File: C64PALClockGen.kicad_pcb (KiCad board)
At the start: 2 copper layers, 21.7 x 32.7 mm, 20 parts, among them J1 Conn_01x08_Pin, J2 Conn_01x08_Pin, U1 74AHCT1G125, U2 LDL1117S33, U3 74AHCT1G125, Y1 5V49EE902

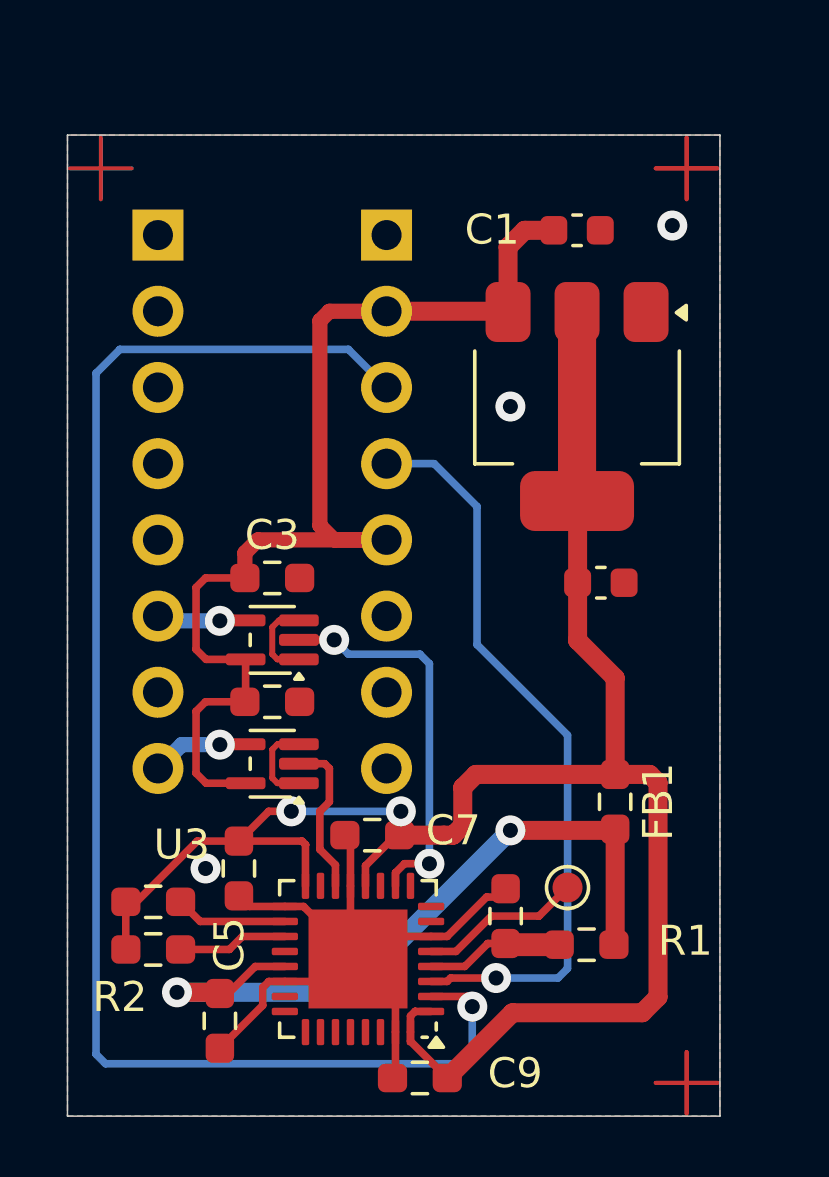
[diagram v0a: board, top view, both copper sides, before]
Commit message: C64 Clock Generator Rev.B
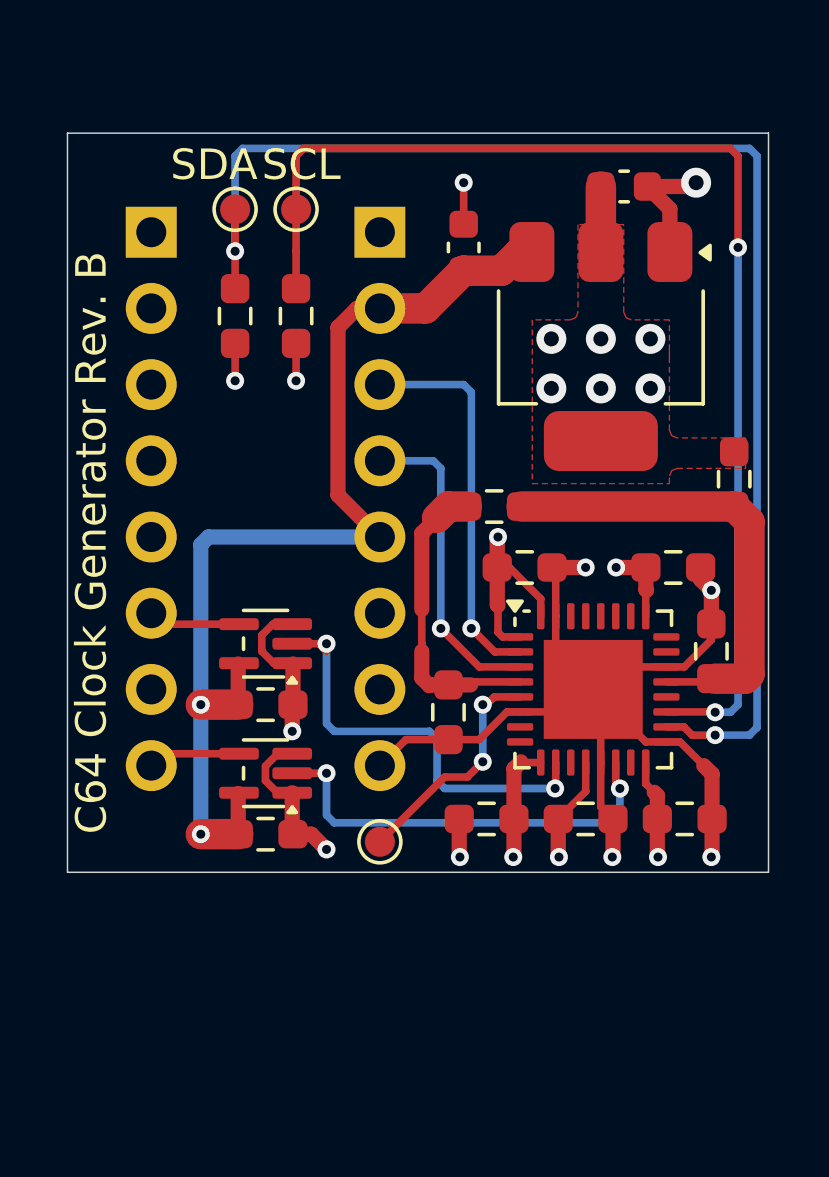
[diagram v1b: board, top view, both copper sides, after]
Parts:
- added C10: 100n, Resistor_SMD:R_0603_1608Metric_Pad0.98x0.95mm_HandSolder, F.Cu at (136.0, 96.4)
- added C11: 100n, Resistor_SMD:R_0603_1608Metric_Pad0.98x0.95mm_HandSolder, F.Cu at (142.2, 88.0)
- added TP2: SDA, TestPoint:TestPoint_Pad_D1.0mm, F.Cu at (127.6, 76.1)
- added TP3: SCL, TestPoint:TestPoint_Pad_D1.0mm, F.Cu at (129.7, 76.1)
- moved R2 21.6 mm to (129.7, 79.7), turned to 90 degrees
- moved C6 20.5 mm to (143.5, 90.8), turned to 90 degrees
- moved R3 19.7 mm to (127.6, 79.7), turned to 90 degrees
- moved R1 14.9 mm to (136.3, 86.0)
- moved C7 13.8 mm to (137.3, 88.0), turned to 0 degrees
- moved C2 13.2 mm to (140.6, 75.3)
- moved C8 12.3 mm to (142.6, 96.4), turned to 0 degrees
- moved Y1 11.9 mm to (139.6, 92.1), turned to 0 degrees
- moved FB1 11.5 mm to (144.3, 85.1)
- moved C3 8.54 mm to (128.6, 96.9)
- moved C9 7.13 mm to (139.3, 96.4), turned to 0 degrees
- moved C5 7.06 mm to (134.7, 92.9), turned to -90 degrees
- moved TP1 6.44 mm to (132.4, 97.2)
- moved C1 3.82 mm to (135.2, 77.4), turned to 90 degrees
- moved U1 2.15 mm to (139.8, 80.7)
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- renumbered C8 to C5, C5 to C6, C10 to C7, C9 to C8, C7 to C9, U2 to U1, U3 to U2, U1 to U3
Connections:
- net /COLCLK renamed COLCLK
- net /COLCLK_UB renamed COLCLK_UB
- net /DOTCLK renamed DOTCLK
- net /DOTCLK_UB renamed DOTCLK_UB
- net /XCLKIN renamed XCLKIN
- net /XIN renamed XIN
- net /XOUT renamed XOUT
- Y1 pad 11: unconnected-(Y1-OUT4B-Pad11) -> (no net)
- Y1 pad 15: unconnected-(Y1-OUT5B-Pad15) -> (no net)
- Y1 pad 20: unconnected-(Y1-CLKSEL-Pad20) -> (no net)
- Y1 pad 23: unconnected-(Y1-OUT6-Pad23) -> (no net)
- Y1 pad 24: unconnected-(Y1-OUT3-Pad24) -> (no net)
- Y1 pad 25: unconnected-(Y1-VDDO3-Pad25) -> +3V3
- Y1 pad 26: unconnected-(Y1-SEL2-Pad26) -> (no net)
- Y1 pad 27: unconnected-(Y1-SEL1-Pad27) -> (no net)
- Y1 pad 28: unconnected-(Y1-SEL0-Pad28) -> (no net)
- Y1 pad 29: unconnected-(Y1-SD/OE-Pad29) -> (no net)
- Y1 pad 30: unconnected-(Y1-OUT0-Pad30) -> (no net)
- Y1 pad 7: unconnected-(Y1-OUT1-Pad7) -> (no net)
- Y1 pad 8: unconnected-(Y1-OUT2-Pad8) -> (no net)
- Y1 pad 9: unconnected-(Y1-VDDO1-Pad9) -> +3V3
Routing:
- net /SDA: track 3.75 -> 45.7 mm, vias 0 -> 2
- net +3V3: track 63.6 -> 24.5 mm, vias 2 -> 13
- net /SCL: track 3.66 -> 40.2 mm, vias 0 -> 2
- net XOUT: track 48.9 -> 13.0 mm
- net (no net): track 33.0 -> 0.00 mm
- net GND: track 32.1 -> 52.5 mm, vias 3 -> 9
- net XIN: track 25.0 -> 10.6 mm
- net COLCLK_UB: track 5.34 -> 14.3 mm, vias 0 -> 2
- net +3V3_Ana: track 24.7 -> 15.8 mm, vias 2 -> 0
- net +3V3_Xtal: track 4.60 -> 10.4 mm
- net XCLKIN: track 5.43 -> 7.66 mm, vias 0 -> 2
- net +5V: track 38.0 -> 36.1 mm, vias 0 -> 2
- net DOTCLK_UB: track 13.0 -> 14.1 mm
- net COLCLK: track 3.26 -> 3.09 mm, vias 1 -> 0
- net DOTCLK: track 2.99 -> 3.07 mm, vias 1 -> 0
- added copper zone on F.Cu, net +3V3
- added copper zone on In2.Cu, net +3V3
- added copper zone on In1.Cu, net GND
- removed copper zone on B.Cu, net GND
- removed copper zone on F.Cu, net GND
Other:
- board size 21.7 x 32.7 mm -> 23.4 x 24.6 mm
- copper layers 2 -> 4
- board text added: "C64 Clock Generator Rev. B"
- board text added: "SCL"
- board text added: "SDA"
